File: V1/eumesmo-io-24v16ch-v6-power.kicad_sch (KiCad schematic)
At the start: 51 parts, among them J6 250-202, J7 USB_C_Receptacle_USB2.0, Q1 WPM2015-3/TR, Q2 MMUN2211LT3G, U1 TX4138, U2 SY8089A1AAC

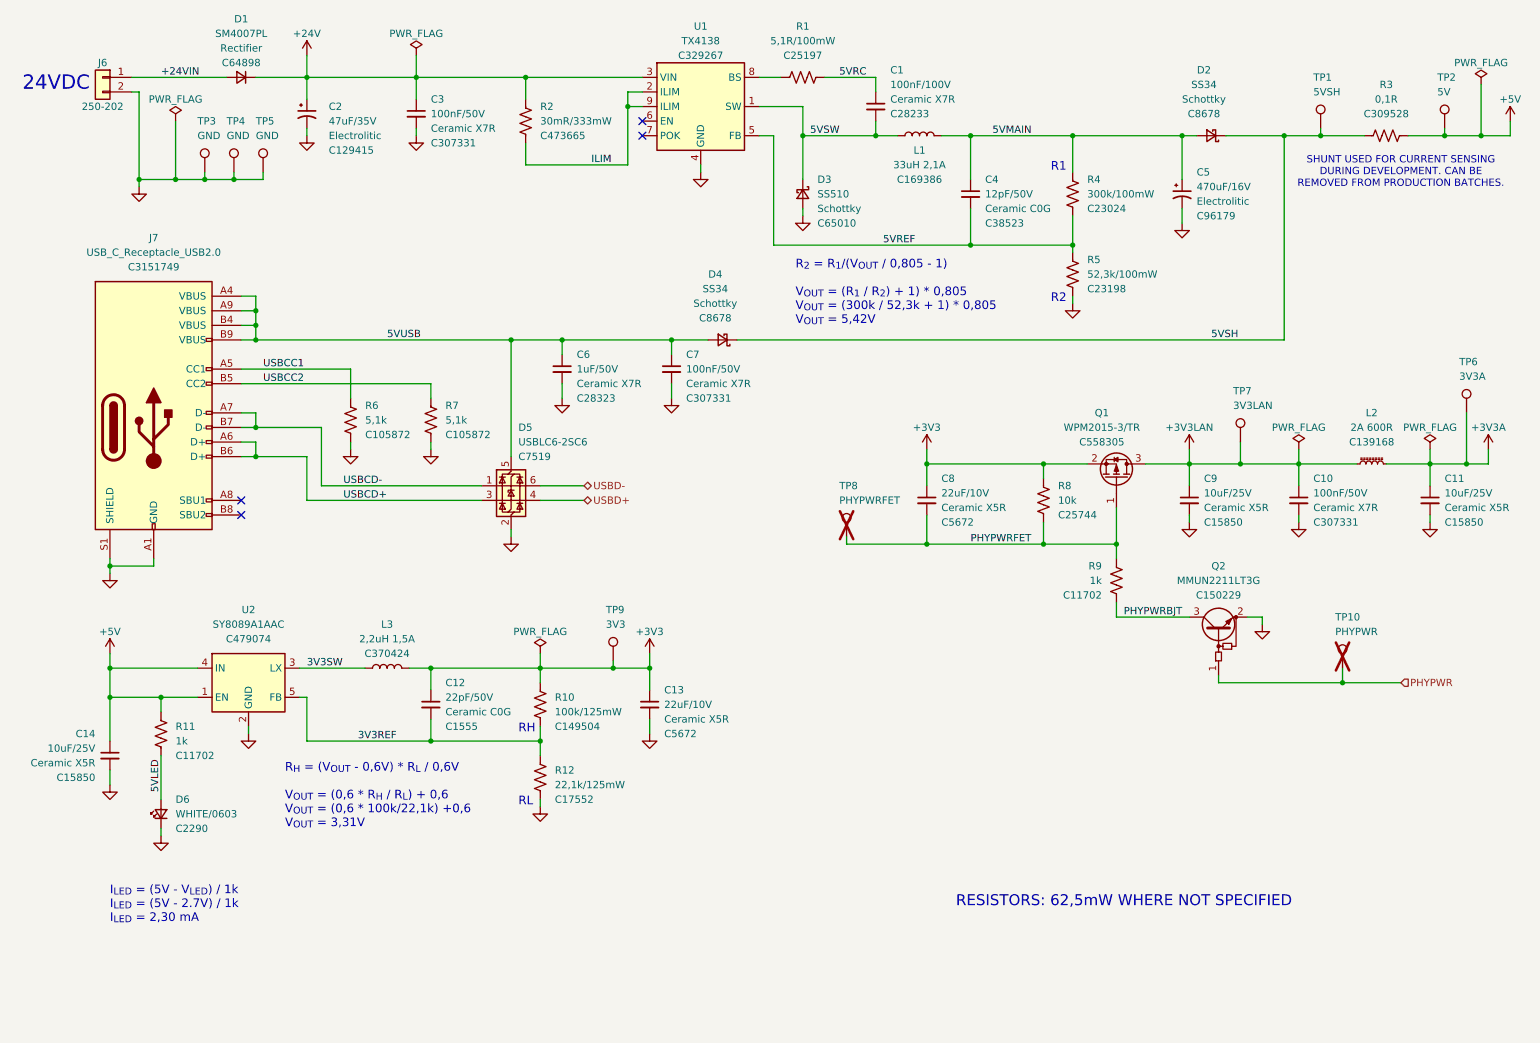
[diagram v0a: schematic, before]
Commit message: Development.
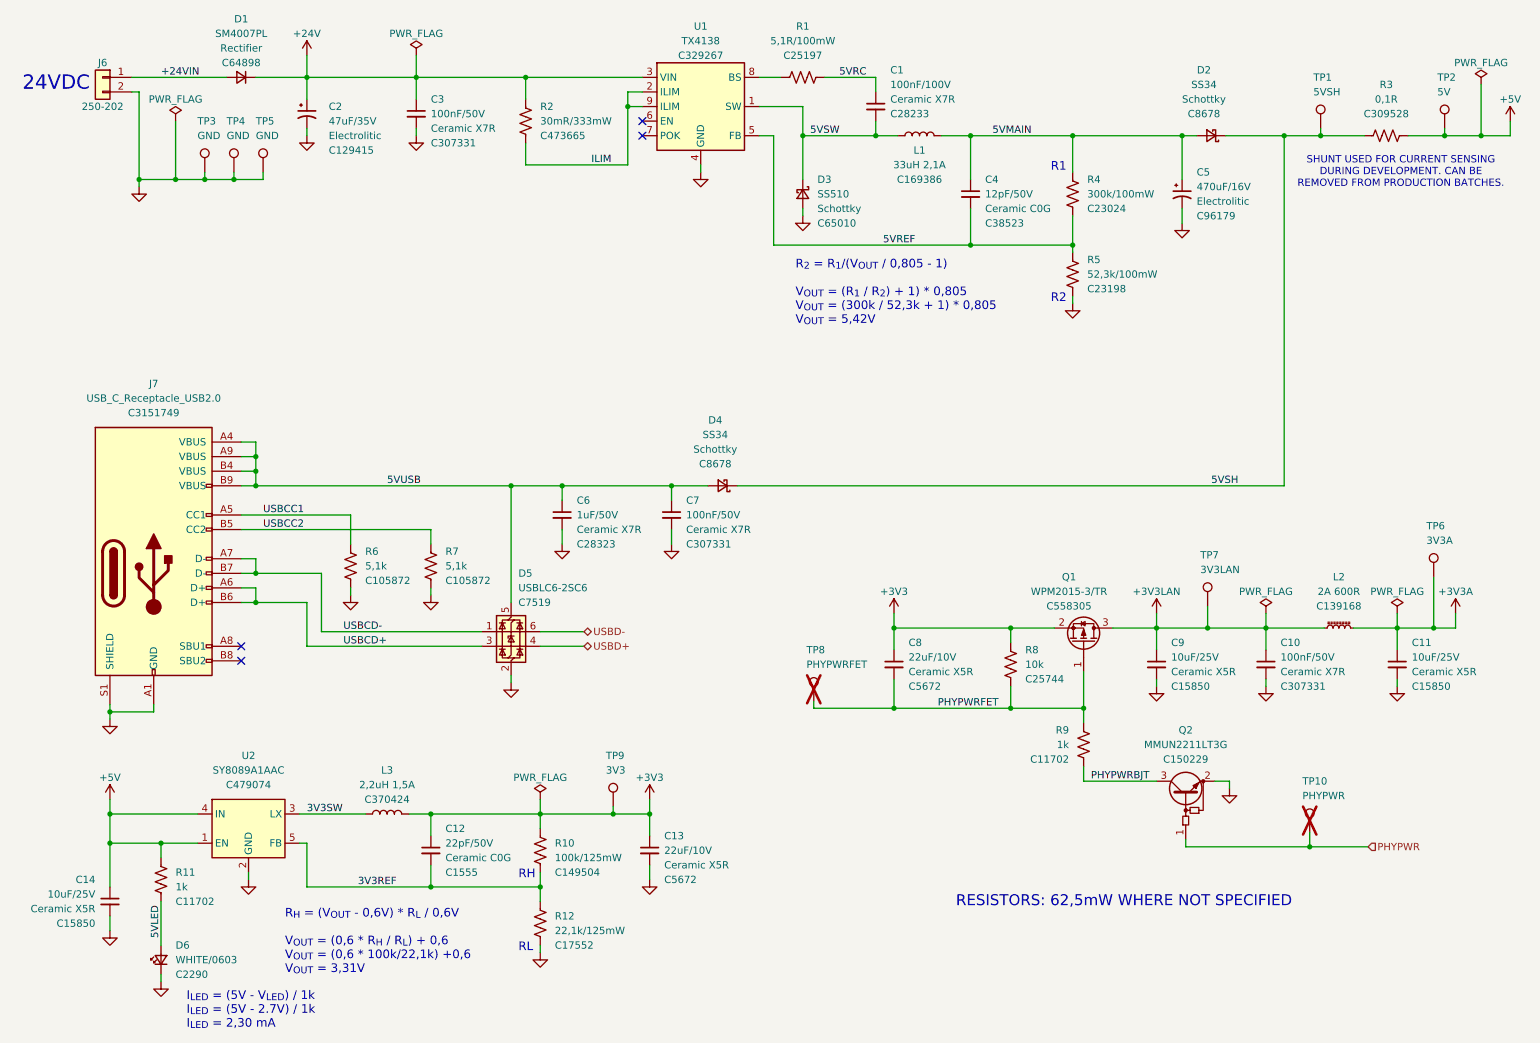
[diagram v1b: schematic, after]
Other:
- moved on the sheet: C10, C11, C12, C13, C14, C6, C7, C8, C9, D4, D5, D6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
